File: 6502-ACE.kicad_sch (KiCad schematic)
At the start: 185 parts, among them J1 PHI2 Select, J10 AUDIO L, J11 DB9 MALE (DTE), J12 PS/2, J13 AUDIO R, J14 AUDIO, J15 5V DC, J16 CART, J17 BUS, J18 VCC, J19 POWER LED, J2 CTS EN, J20 STORAGE, J3 RESET SW, J4 DCD EN, J5 JOYSTICK A, J6 PADDLES, J7 JOYSTICK B, J8 PORT B, J9 PORT A, SW1 `, SW10 9, SW11 0, SW12 -, SW13 =, SW14 BACKSPACE, SW15 ESCAPE, SW16 TAB, SW17 Q, SW18 W, SW19 E, SW2 1, SW20 R, SW21 T, SW22 Y, SW23 U, SW24 I, SW25 O, SW26 P, SW27 [, SW28 ], SW29 \, SW3 2, SW30 INSERT, SW31 CAPS LOCK, SW32 A, SW33 S, SW34 D, SW35 F, SW36 G, SW37 H, SW38 J, SW39 K, SW4 3, SW40 L, SW41 SHIFT, SW42 ;, SW43 ', SW44 ENTER, SW45 DELETE, SW46 Z, SW47 X, SW48 C, SW49 R SHIFT, SW5 4, SW50 V, SW51 B, SW52 N, SW53 M, SW54 ,, SW55 ., SW56 /, SW57 UP ARROW, SW58 CTRL, SW59 ALT, SW6 5, SW60 MENU, SW61 SPACE, SW62 FN, SW63 LEFT ARROW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

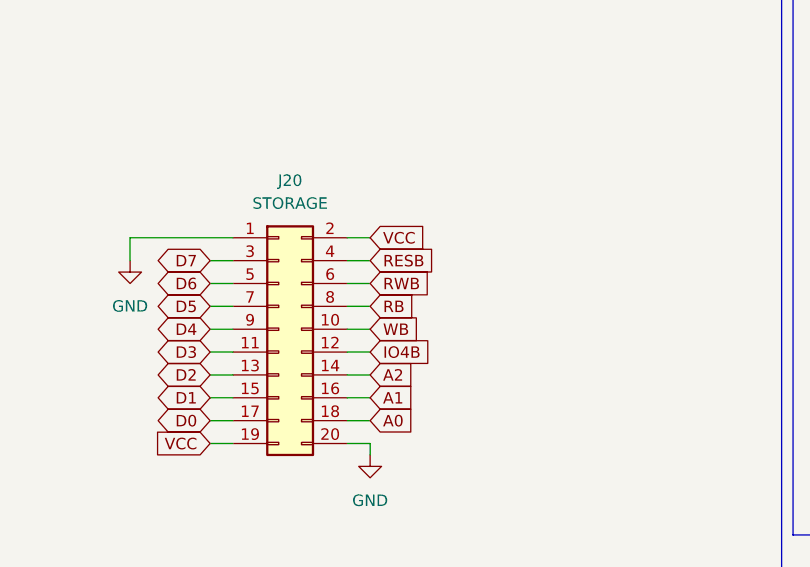
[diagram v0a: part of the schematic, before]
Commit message: Change headers
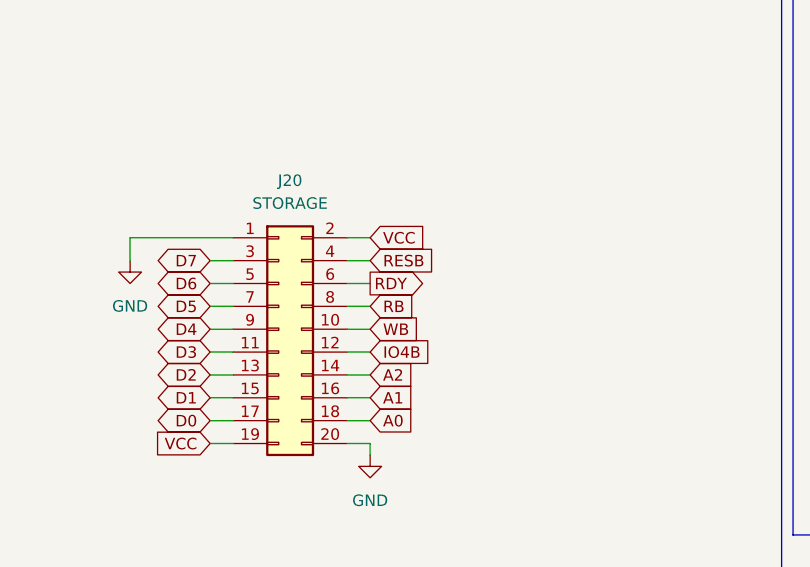
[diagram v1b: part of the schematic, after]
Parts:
- J14, J18, J19, J3: footprint Connector_JST:JST_XH_B2B-XH-A_1x02_P2.50mm_Vertical -> Connector_PinHeader_2.54mm:PinHeader_1x02_P2.54mm_Vertical
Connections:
- net RDY: now also J20.6 (Pin_6)
- net RWB: no longer J20.6 (Pin_6)
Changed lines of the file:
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@@
 		)
 	)
-	(global_label "RWB"
-		(shape input)
+	(global_label "RDY"
+		(shape output)
 		(at 534.67 346.71 0)
 		(effects
@@
 			)
 		)
-		(property "Footprint" "Connector_JST:JST_XH_B2B-XH-A_1x02_P2.50mm_Vertical"
+		(property "Footprint" "Connector_PinHeader_2.54mm:PinHeader_1x02_P2.54mm_Vertical"
 			(at 637.54 260.35 0)
 			(hide yes)
@@
 			)
 		)
-		(property "Footprint" "Connector_JST:JST_XH_B2B-XH-A_1x02_P2.50mm_Vertical"
+		(property "Footprint" "Connector_PinHeader_2.54mm:PinHeader_1x02_P2.54mm_Vertical"
 			(at 374.65 88.9 0)
 			(hide yes)
@@
 			)
 		)
-		(property "Footprint" "Connector_JST:JST_XH_B2B-XH-A_1x02_P2.50mm_Vertical"
+		(property "Footprint" "Connector_PinHeader_2.54mm:PinHeader_1x02_P2.54mm_Vertical"
 			(at 637.54 274.32 0)
 			(hide yes)
@@
 			)
 		)
-		(property "Footprint" "Connector_JST:JST_XH_B2B-XH-A_1x02_P2.50mm_Vertical"
+		(property "Footprint" "Connector_PinHeader_2.54mm:PinHeader_1x02_P2.54mm_Vertical"
 			(at 412.75 201.93 0)
 			(hide yes)
